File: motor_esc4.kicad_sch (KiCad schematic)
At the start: 14 parts, among them J11 SolderWirePad_1x01_SMD_3x6mm, J12 SolderWirePad_1x01_SMD_3x6mm, J13 SolderWirePad_1x01_SMD_3x6mm, U7 MCF8316A

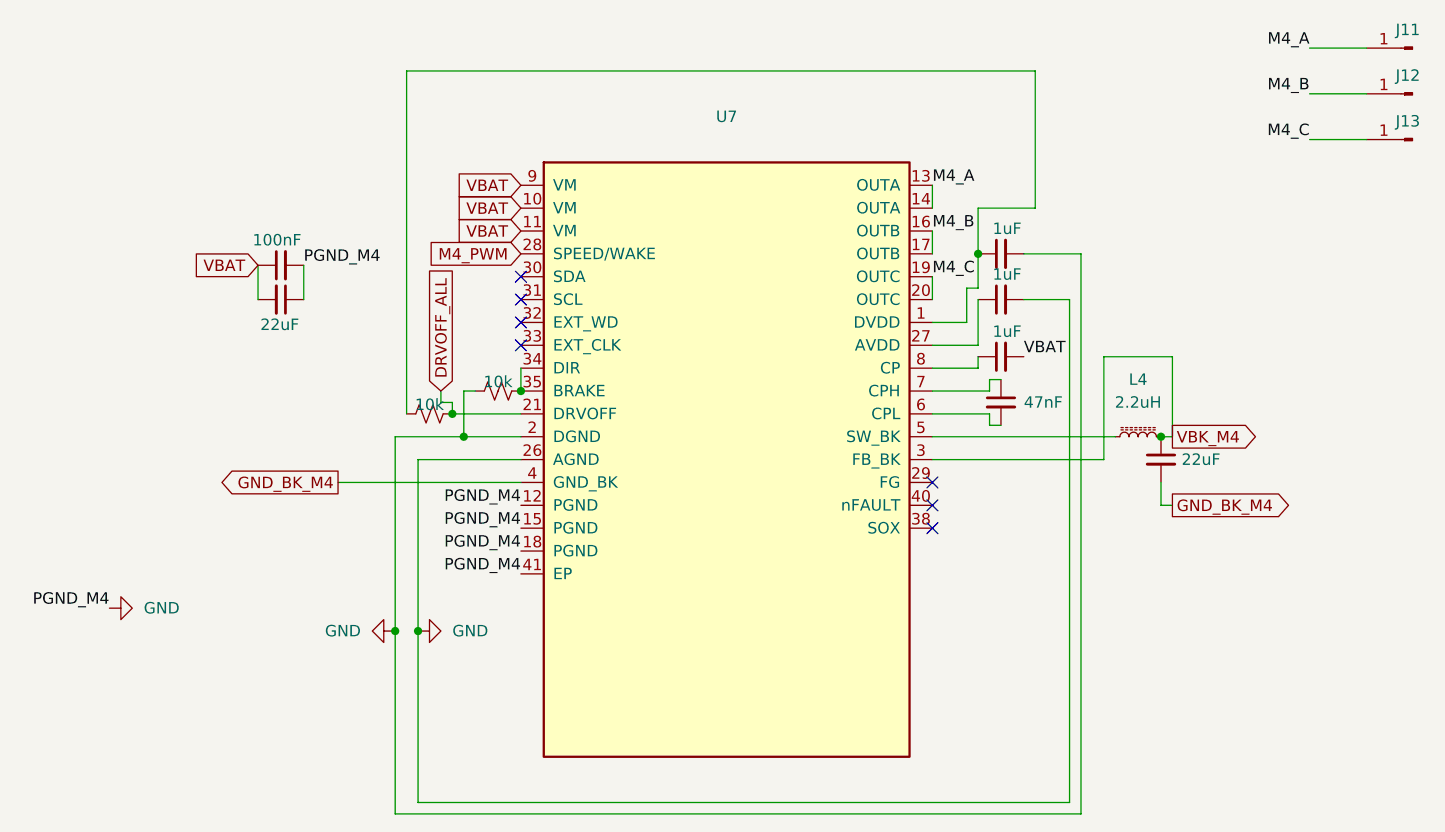
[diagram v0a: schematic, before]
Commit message: done?
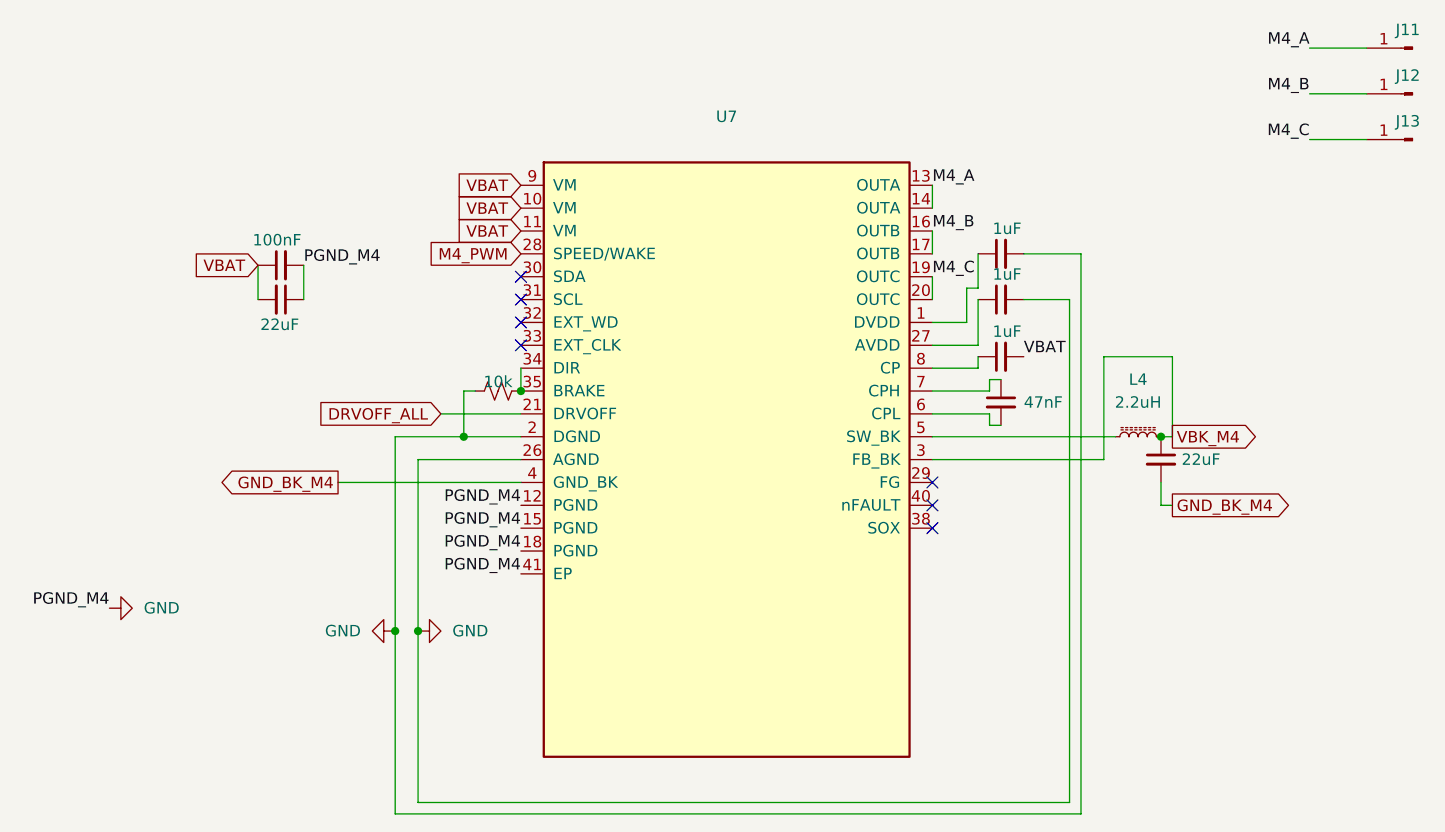
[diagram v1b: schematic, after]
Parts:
- removed R13: 10k, Resistor_SMD:R_0603_1608Metric_Pad0.98x0.95mm_HandSolder, symbol Device:R_Small_US
- R15: footprint Resistor_SMD:R_0603_1608Metric_Pad0.98x0.95mm_HandSolder -> Resistor_SMD:R_0402_1005Metric_Pad0.72x0.64mm_HandSolder
